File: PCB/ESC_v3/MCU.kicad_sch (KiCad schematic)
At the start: 44 parts, among them J10 Conn_01x01_Pin, J3 Conn_01x01_Pin, J4 Conn_01x01_Pin, J5 Conn_01x01_Pin, J6 Conn_01x01_Pin, J7 Conn_01x01_Pin, J8 Conn_01x01_Pin, J9 Conn_01x01_Pin, U3 STM32G474CETx, Y2 24MHz

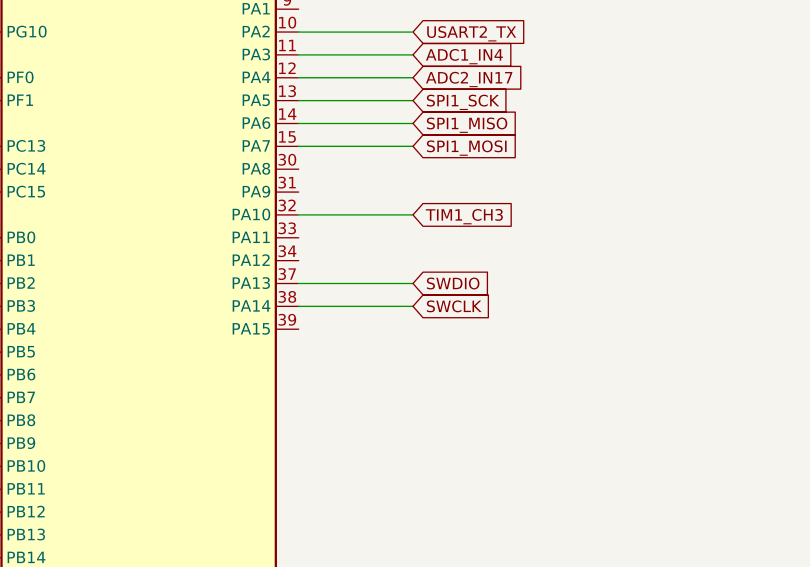
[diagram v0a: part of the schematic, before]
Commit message: Layout edit
Changed some layout and optimized
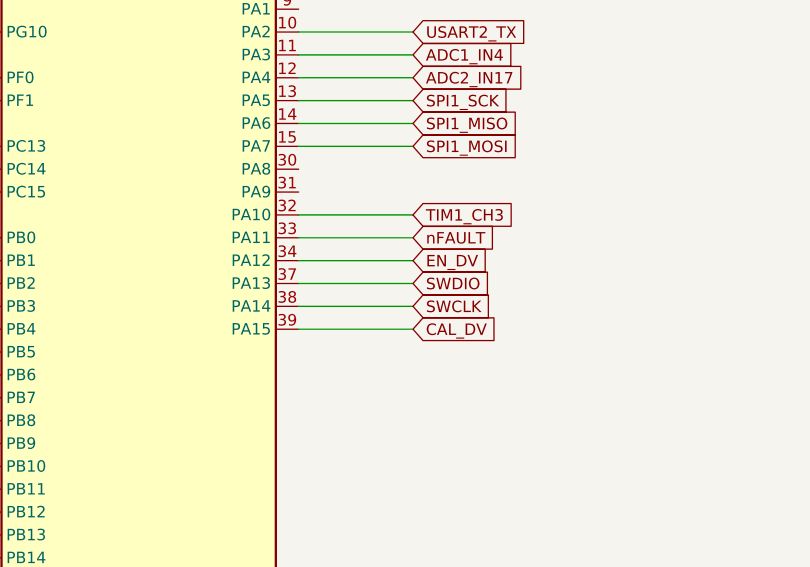
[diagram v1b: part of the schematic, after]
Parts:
- C24: footprint Capacitor_SMD:C_0805_2012Metric -> Capacitor_SMD:C_0603_1608Metric
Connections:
- net CAL_DV: now also U3.39 (PA15)
- net EN_DV: now also U3.34 (PA12)
- net nFAULT: now reaches U3.33 (PA11)
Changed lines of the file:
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@@
 	(wire
 		(pts
+			(xy 154.94 106.68) (xy 167.64 106.68)
+		)
+		(stroke
+			(width 0)
+			(type default)
+		)
+	)
+	(wire
+		(pts
 			(xy 137.16 67.31) (xy 137.16 68.58)
 		)
@@
 	(wire
 		(pts
+			(xy 167.64 104.14) (xy 154.94 104.14)
+		)
+		(stroke
+			(width 0)
+			(type default)
+		)
+	)
+	(wire
+		(pts
 			(xy 92.71 46.99) (xy 92.71 53.34)
 		)
@@
 	(wire
 		(pts
+			(xy 154.94 114.3) (xy 167.64 114.3)
+		)
+		(stroke
+			(width 0)
+			(type default)
+		)
+	)
+	(wire
+		(pts
 			(xy 167.64 101.6) (xy 154.94 101.6)
 		)
@@
 		)
 	)
+	(global_label "CAL_DV"
+		(shape input)
+		(at 167.64 114.3 0)
+		(fields_autoplaced yes)
+		(effects
+			(font
+				(size 1.27 1.27)
+				(thickness 0.1588)
+			)
+			(justify left)
+		)
+		(property "Intersheetrefs" "${INTERSHEET_REFS}"
+			(at 177.3381 114.3 0)
+			(effects
+				(font
+					(size 1.27 1.27)
+				)
+				(justify left)
+				(hide yes)
+			)
+		)
+	)
 	(global_label "EN_DV"
 		(shape input)
@@
 		)
 	)
+	(global_label "nFAULT"
+		(shape input)
+		(at 167.64 104.14 0)
+		(fields_autoplaced yes)
+		(effects
+			(font
+				(size 1.27 1.27)
+				(thickness 0.1588)
+			)
+			(justify left)
+		)
+		(property "Intersheetrefs" "${INTERSHEET_REFS}"
+			(at 177.7536 104.14 0)
+			(effects
+				(font
+					(size 1.27 1.27)
+				)
+				(justify left)
+				(hide yes)
+			)
+		)
+	)
 	(global_label "ADC2_IN17"
 		(shape input)
@@
 		)
 	)
+	(global_label "EN_DV"
+		(shape input)
+		(at 167.64 106.68 0)
+		(fields_autoplaced yes)
+		(effects
+			(font
+				(size 1.27 1.27)
+				(thickness 0.1588)
+			)
+			(justify left)
+		)
+		(property "Intersheetrefs" "${INTERSHEET_REFS}"
+			(at 176.4309 106.68 0)
+			(effects
+				(font
+					(size 1.27 1.27)
+				)
+				(justify left)
+				(hide yes)
+			)
+		)
+	)
 	(global_label "INHA"
 		(shape input)
@@
 			)
 		)
-		(property "Footprint" "Capacitor_SMD:C_0805_2012Metric"
+		(property "Footprint" "Capacitor_SMD:C_0603_1608Metric"
 			(at 34.5948 53.34 0)
 			(effects
